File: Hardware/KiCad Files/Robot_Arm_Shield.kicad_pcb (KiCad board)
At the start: 2 copper layers, 29 parts, among them P1 Power Input, P14 Power Jumper, U1 LM 7805

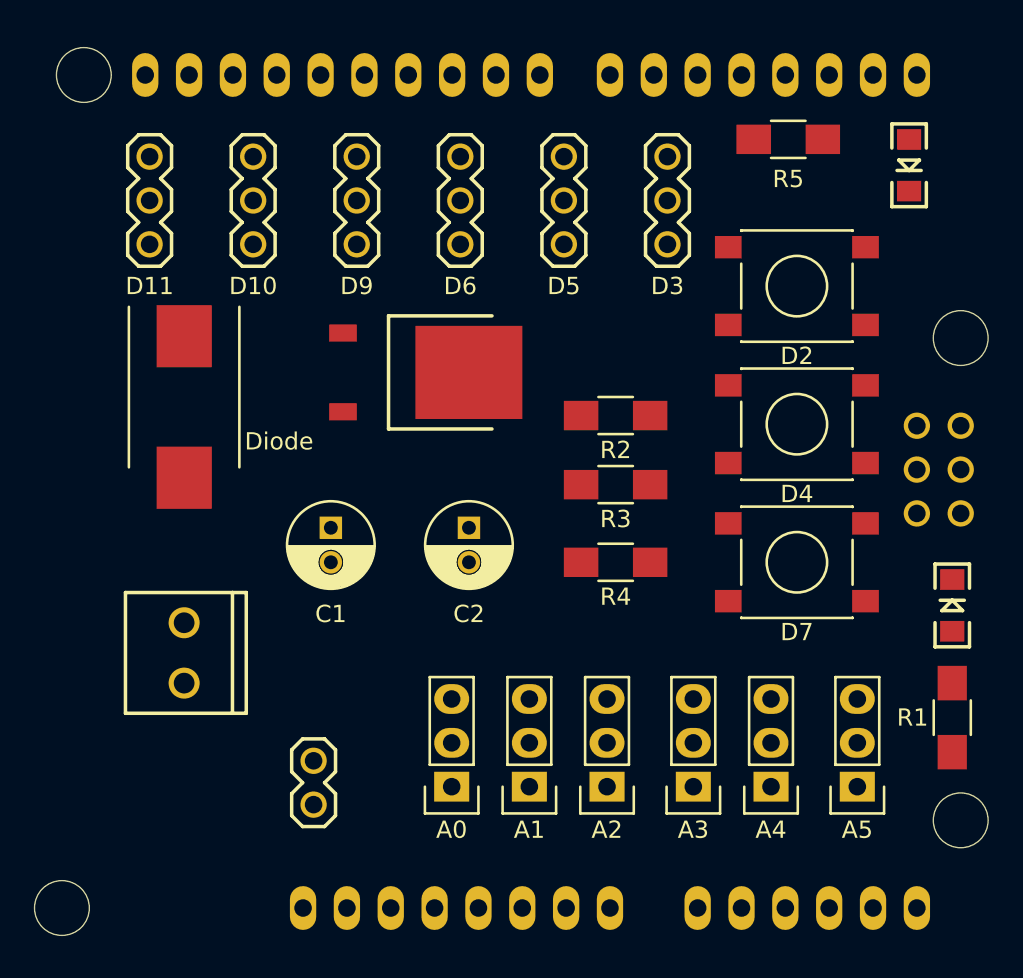
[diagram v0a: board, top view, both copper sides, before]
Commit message: Finalized Board. Exported Gerbers
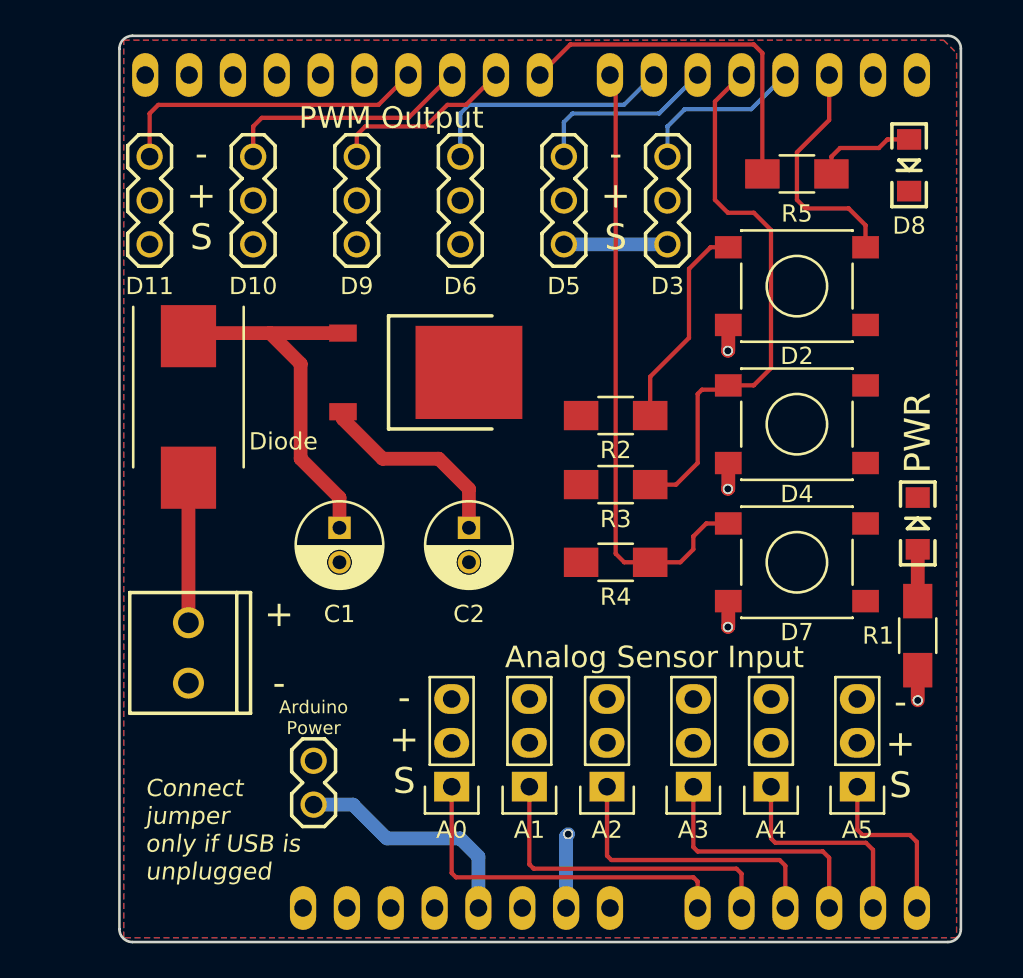
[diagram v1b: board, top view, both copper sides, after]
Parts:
- added REF**: Symbol_OSHW-Logo_SilkScreen, Symbols:Symbol_OSHW-Logo_SilkScreen, B.Cu at (113.2, 101.2)
- moved LED1 5.15 mm to (153.0, 86.2)
- moved R1 5.15 mm to (153.0, 92.8)
- moved R5 2.06 mm to (146.0, 66.0)
- moved C1 0.50 mm to (119.5, 86.5)
- moved Diode 0.25 mm to (110.8, 79.5)
- moved P1 0.25 mm to (110.8, 95.5)
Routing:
- net /SW2: track 0.00 -> 36.0 mm
- net /SW1: track 0.00 -> 32.0 mm
- net /SW0: track 0.00 -> 26.1 mm
- net Net-(C1-Pad1): track 0.00 -> 22.2 mm
- net /A0: track 0.00 -> 21.0 mm
- net /LED0: track 0.00 -> 20.8 mm
- net /A1: track 0.00 -> 19.5 mm
- net /PWM5: track 0.00 -> 18.4 mm
- net /5V: track 0.00 -> 17.9 mm, vias 0 -> 4
- net /A2: track 0.00 -> 17.0 mm
- net /A3: track 0.00 -> 15.4 mm
- net /PWM2: track 0.00 -> 15.2 mm
- net /PWM4: track 0.00 -> 14.5 mm
- net Net-(P14-Pad2): track 0.00 -> 13.8 mm
- net /A4: track 0.00 -> 12.6 mm
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- added copper zone on B.Cu, net /5V
- added copper zone on F.Cu, net GND
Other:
- board outline added: 48.8 x 52.5 mm
- net class Power added: clearance 0.2, trace_width 0.8, via_dia 0.6, via_drill 0.4
- board text added: "+"
- board text added: "-"
- board text added: "- + S"
- board text added: "Analog Sensor Input"
- board text added: "Arduino Power"
- board text added: "Connect jumper only if USB is unplugged"
- board text added: "D8"
- board text added: "PWM Output"
- board text added: "PWR"
- board text added: "Robot Arm Control Shield Designed By: Cole Mortensen, 2016 Revision: 1.0"
